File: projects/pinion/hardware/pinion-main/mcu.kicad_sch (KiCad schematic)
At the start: 1 part, among them U1 STM32H753VIHx

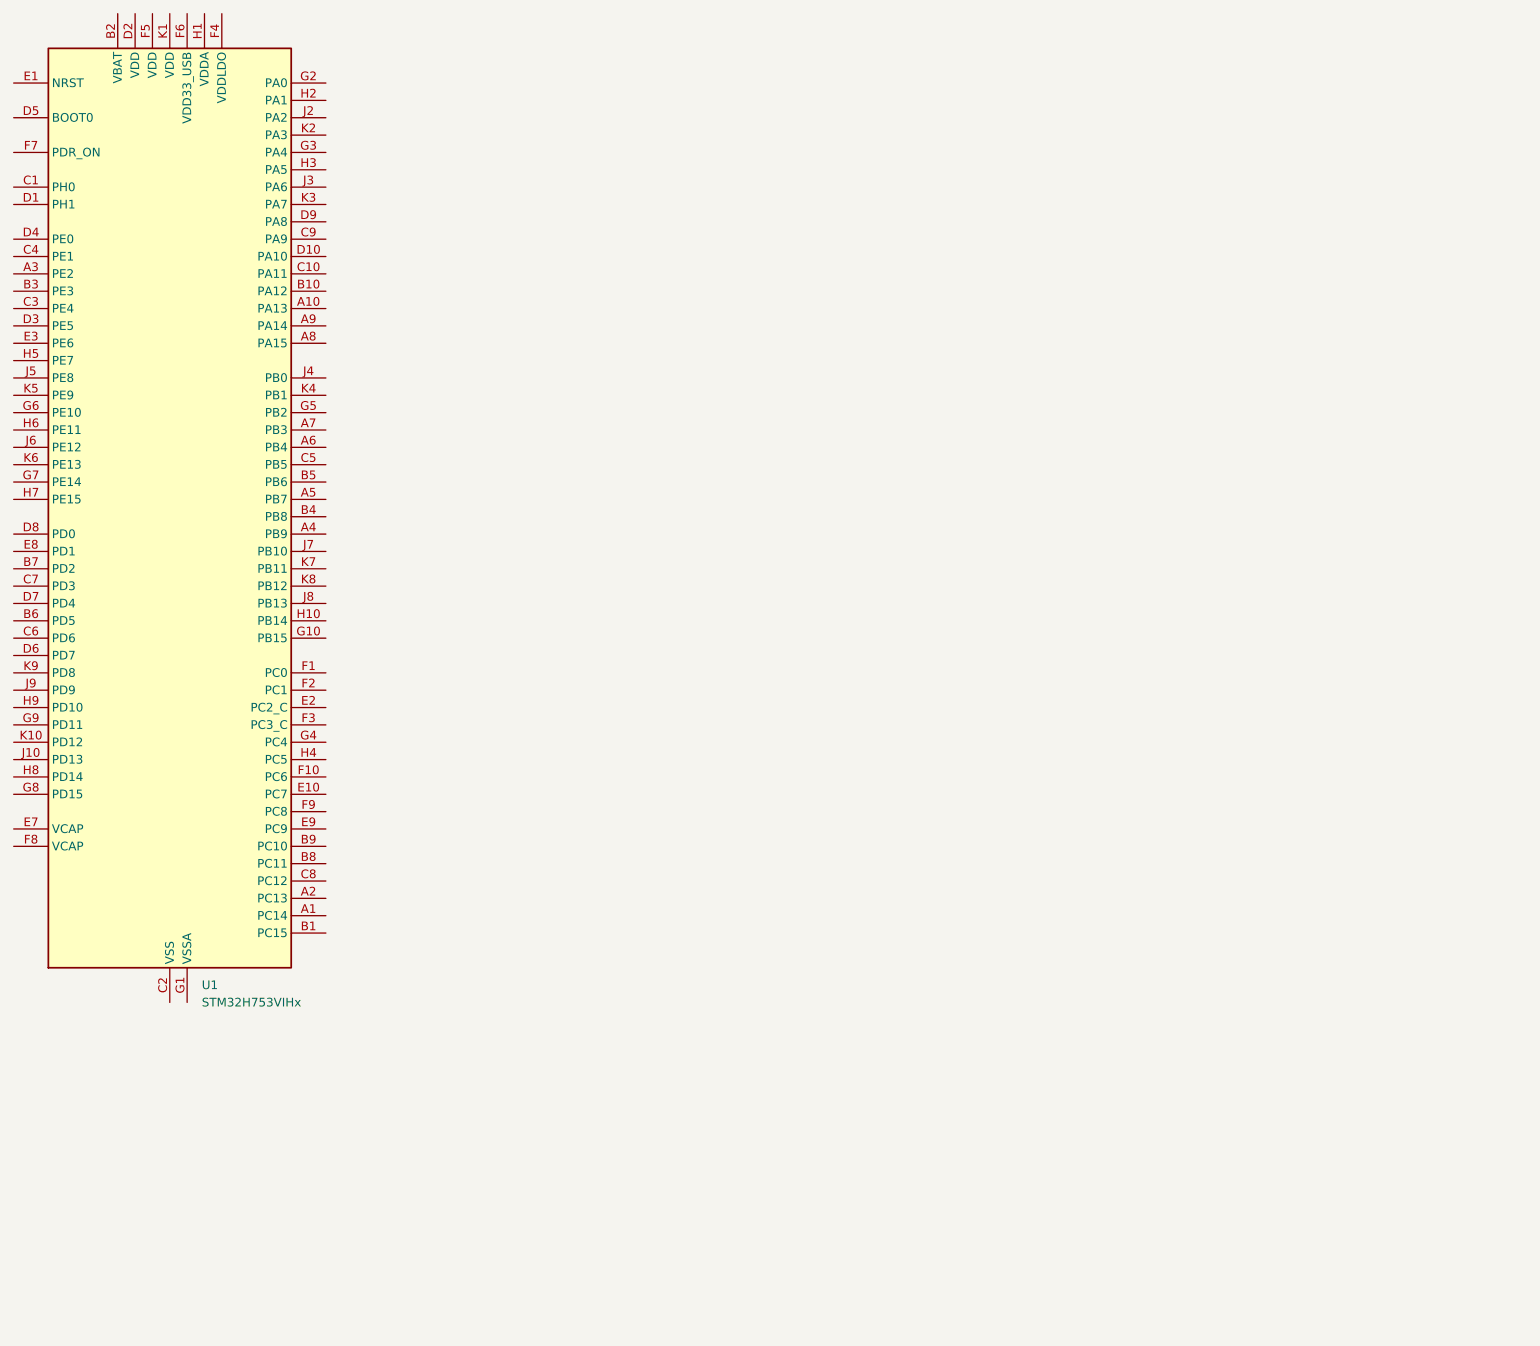
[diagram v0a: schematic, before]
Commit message: [pinion] mcu basic schematic in
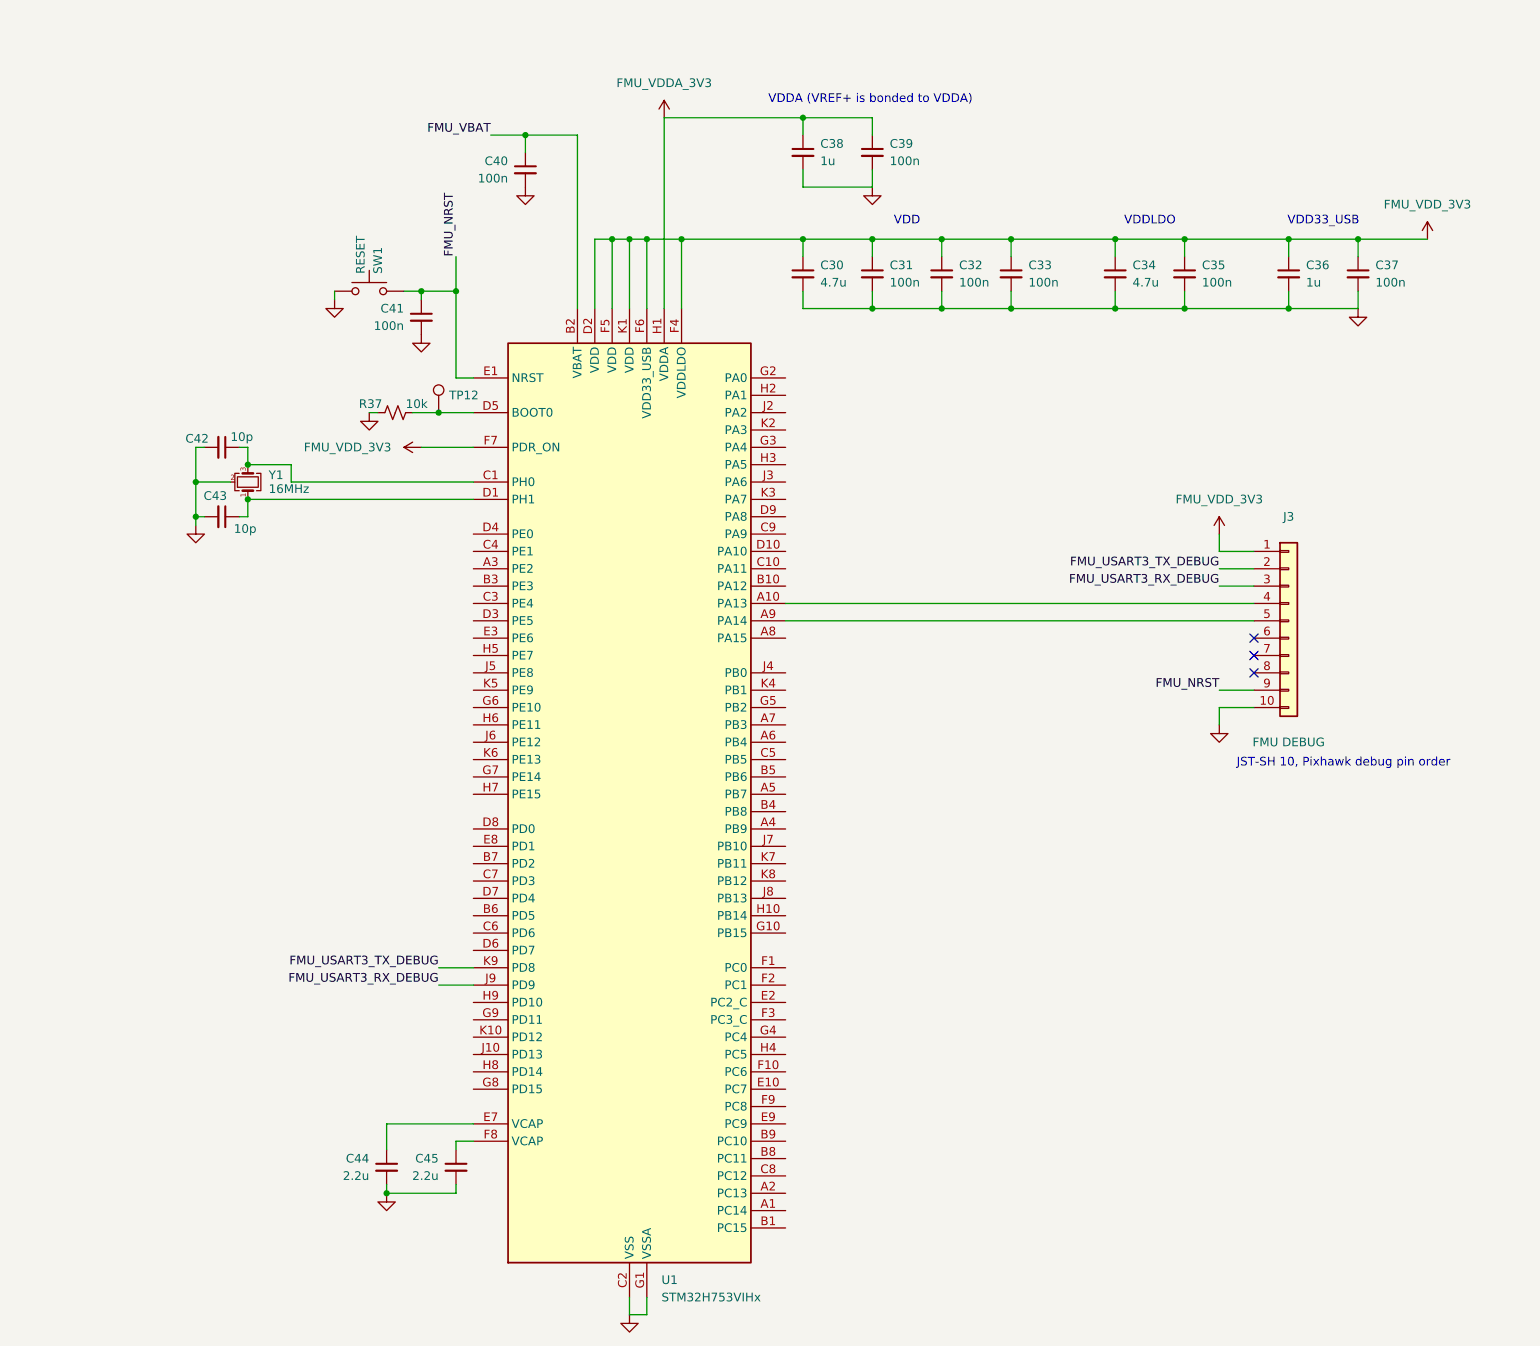
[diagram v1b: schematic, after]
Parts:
- added C30, C34: 4.7u, Capacitor_SMD:C_0603_1608Metric, symbol Device:C_Small
- added C31, C32, C33, C35, C37, C39, C40, C41: 100n, Capacitor_SMD:C_0402_1005Metric, symbol Device:C_Small
- added C36, C38: 1u, Capacitor_SMD:C_0402_1005Metric, symbol Device:C_Small
- added C42, C43: 10p, Capacitor_SMD:C_0402_1005Metric, symbol Device:C_Small
- added C44, C45: 2.2u, Capacitor_SMD:C_0603_1608Metric, symbol Device:C_Small
- added J3: FMU DEBUG, Connector_JST:JST_SH_SM10B-SRSS-TB_1x10-1MP_P1.00mm_Horizontal, symbol Connector_Generic:Conn_01x10
- added R37: 10k, Resistor_SMD:R_0402_1005Metric, symbol Device:R_Small_US
- added SW1: RESET, Button_Switch_SMD:SW_SPST_B3U-1000P, symbol Switch:SW_Push
- added TP12: TestPoint, TestPoint:TestPoint_Pad_D1.0mm, symbol Connector:TestPoint
- added Y1: 16MHz, Crystal:Crystal_SMD_3225-4Pin_3.2x2.5mm, symbol Device:Crystal_GND24_Small
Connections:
- net at U1.A10 (PA13): now also J3.4 (Pin_4)
- net at U1.A9 (PA14): now also J3.5 (Pin_5)
- net FMU_VBAT: now reaches U1.B2 (VBAT)
- net FMU_VBAT: now also C40.1
- net at U1.C1 (PH0): now also C42.1, Y1.3
- net GND: now reaches U1.C2 (VSS), U1.E4 (VSS), U1.E5 (VSS), U1.E6 (VSS), U1.J1 (VSS)
- net GND: now also U1.G1 (VSSA), C30.2, C31.2, C32.2, C33.2, C34.2, C35.2, C36.2, C37.2, C38.2, C39.2, C40.2, C41.2, C42.2, C43.2, C44.2, C45.2, J3.10 (Pin_10), R37.2, SW1.1, Y1.2 (G), Y1.4 (G)
- net at U1.D1 (PH1): now also C43.1, Y1.1
- net FMU_VDD_3V3: now reaches U1.D2 (VDD)
- net FMU_VDD_3V3: now also U1.F4 (VDDLDO), U1.F5 (VDD), U1.F6 (VDD33_USB), U1.F7 (PDR_ON), U1.K1 (VDD), C30.1, C31.1, C32.1, C33.1, C34.1, C35.1, C36.1, C37.1, J3.1 (Pin_1)
- net at U1.D5 (BOOT0): now also R37.1, TP12.1
- net FMU_NRST: now reaches U1.E1 (NRST)
- net FMU_NRST: now also C41.1, J3.9 (Pin_9), SW1.2
- net at U1.E7 (VCAP): now also C44.1
- net at U1.F8 (VCAP): now also C45.1
- net FMU_VDDA_3V3: now reaches U1.H1 (VDDA)
- net FMU_VDDA_3V3: now also C38.1, C39.1
- net FMU_USART3_RX_DEBUG: now reaches U1.J9 (PD9)
- net FMU_USART3_RX_DEBUG: now also J3.3 (Pin_3)
- net FMU_USART3_TX_DEBUG: now reaches U1.K9 (PD8)
- net FMU_USART3_TX_DEBUG: now also J3.2 (Pin_2)
- no-connect marks 0 -> 3
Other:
- note added: "JST-SH 10, Pixhawk debug pin order"
- note added: "VDD"
- note added: "VDD33_USB"
- note added: "VDDA (VREF+ is bonded to VDDA)"
- note added: "VDDLDO"
- moved on the sheet: U1
